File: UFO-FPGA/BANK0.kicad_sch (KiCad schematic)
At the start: 7 parts, among them U1 ICE40HX8K-BG121

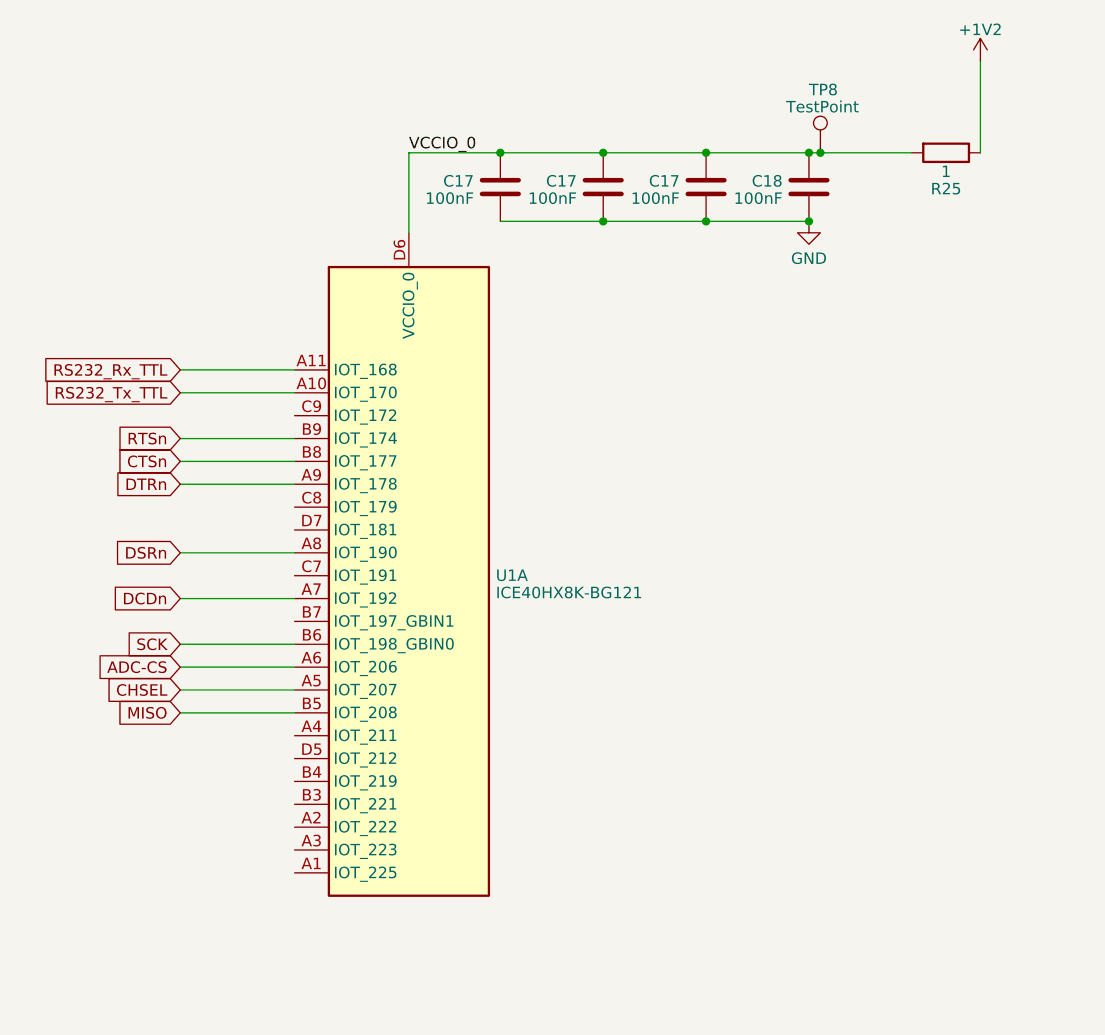
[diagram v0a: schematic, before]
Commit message: IO and power
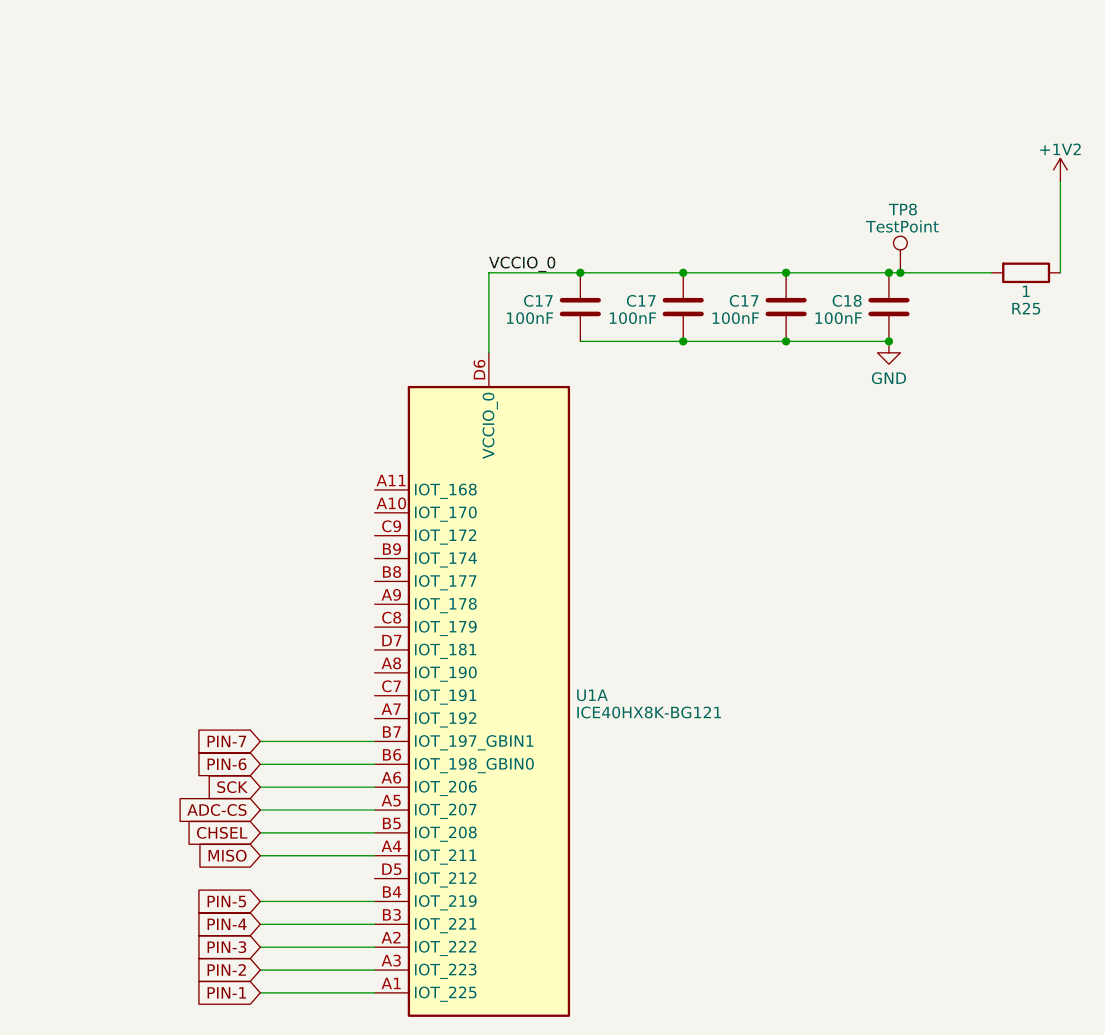
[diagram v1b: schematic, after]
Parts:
- removed C17 (x3): 100nF, symbol Device:C
- added C17 (x3): 100nF, symbol Device:C
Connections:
- net ADC-CS: now also U1.A5 (IOT_207); no longer U1.A6 (IOT_206)
- net CHSEL: now also U1.B5 (IOT_208); no longer U1.A5 (IOT_207)
- net GND: now also C17.2, C17.2, C17.2
- net MISO: now also U1.A4 (IOT_211); no longer U1.B5 (IOT_208)
- net SCK: now also U1.A6 (IOT_206); no longer U1.B6 (IOT_198_GBIN0)
- net VCCIO_0: now also C17.1, C17.1, C17.1
- net PIN-1: now reaches U1.A1 (IOT_225)
- net PIN-3: now reaches U1.A2 (IOT_222)
- net PIN-2: now reaches U1.A3 (IOT_223)
- net PIN-4: now reaches U1.B3 (IOT_221)
- net PIN-5: now reaches U1.B4 (IOT_219)
- net PIN-7: now reaches U1.B7 (IOT_197_GBIN1)
- net CTSn: no longer names the net of U1.B8 (IOT_177)
- net DCDn: no longer names the net of U1.A7 (IOT_192)
- net DSRn: no longer names the net of U1.A8 (IOT_190)
- net DTRn: no longer names the net of U1.A9 (IOT_178)
- net RS232_Rx_TTL: no longer names the net of U1.A11 (IOT_168)
- net RS232_Tx_TTL: no longer names the net of U1.A10 (IOT_170)
- net RTSn: no longer names the net of U1.B9 (IOT_174)
- new net PIN-6: U1.B6 (IOT_198_GBIN0)

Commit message: Revision
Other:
- company: (none) -> Universal-Field-Objects
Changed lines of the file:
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@@
   (paper "A4")
   (title_block
-    (date "2023-04-22")
-    (rev "V0.1")
+    (date "2023-04-25")
+    (rev "V0.5")
+    (company "Universal-Field-Objects")
   )
   (junction (at 160.02 48.895) (diameter 0) (color 0 0 0 0)

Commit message: footprints and PCB
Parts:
- R25: footprint (none) -> Resistor_SMD:R_0805_2012Metric_Pad1.20x1.40mm_HandSolder
- TP8: footprint (none) -> TestPoint:TestPoint_Keystone_5000-5004_Miniature
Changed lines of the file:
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@@
       (effects (font (size 1.27 1.27)) (justify left))
     )
-    (property "Footprint" "" (at 177.8 48.895 0)
+    (property "Footprint" "TestPoint:TestPoint_Keystone_5000-5004_Miniature" (at 177.8 48.895 0)
       (effects (font (size 1.27 1.27)) hide)
     )
@@
       (effects (font (size 1.27 1.27)))
     )
-    (property "Footprint" "" (at 186.69 47.117 90)
+    (property "Footprint" "Resistor_SMD:R_0805_2012Metric_Pad1.20x1.40mm_HandSolder" (at 186.69 47.117 90)
       (effects (font (size 1.27 1.27)) hide)
     )

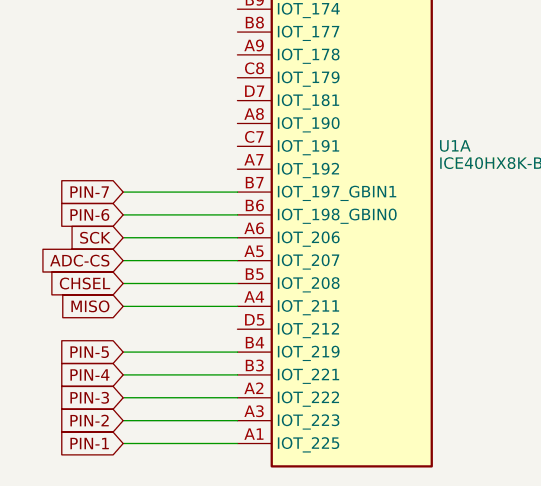
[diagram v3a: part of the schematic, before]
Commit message: footprint
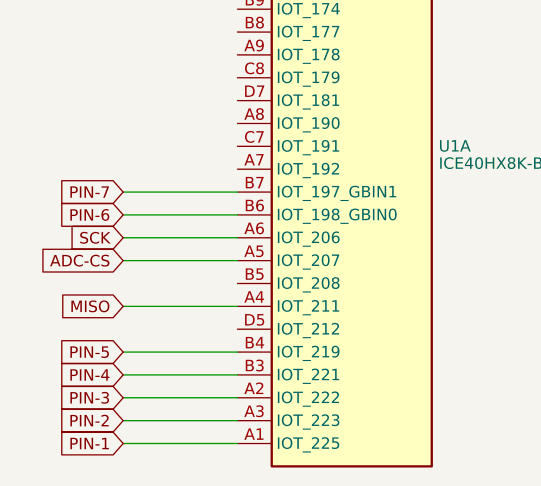
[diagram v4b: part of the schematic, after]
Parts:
- C17, C18: footprint (none) -> Capacitor_SMD:C_0805_2012Metric_Pad1.18x1.45mm_HandSolder
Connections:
- net CHSEL: no longer names the net of U1.B5 (IOT_208)
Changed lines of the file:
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@@
-    (stroke (width 0) (type default))
-  )
-  (wire (pts (xy 101.6 111.125) (xy 114.3 111.125))
     (stroke (width 0) (type default))
   )
@@
     )
   )
-  (global_label "CHSEL" (shape input) (at 101.6 111.125 180) (fields_autoplaced)
-    (effects (font (size 1.27 1.27)) (justify right))
-    (property "Intersheetrefs" "${INTERSHEET_REFS}" (at 92.7071 111.125 0)
-      (effects (font (size 1.27 1.27)) (justify right) hide)
-    )
-  )
   (global_label "PIN-2" (shape input) (at 101.6 126.365 180) (fields_autoplaced)
     (effects (font (size 1.27 1.27)) (justify right))
@@
       (effects (font (size 1.27 1.27)) (justify left))
     )
-    (property "Footprint" "" (at 147.6248 56.515 0)
+    (property "Footprint" "Capacitor_SMD:C_0805_2012Metric_Pad1.18x1.45mm_HandSolder" (at 147.6248 56.515 0)
       (effects (font (size 1.27 1.27)) hide)
     )
@@
       (effects (font (size 1.27 1.27)) (justify left))
     )
-    (property "Footprint" "" (at 159.0548 56.515 0)
+    (property "Footprint" "Capacitor_SMD:C_0805_2012Metric_Pad1.18x1.45mm_HandSolder" (at 159.0548 56.515 0)
       (effects (font (size 1.27 1.27)) hide)
     )
@@
       (effects (font (size 1.27 1.27)) (justify left))
     )
-    (property "Footprint" "" (at 170.4848 56.515 0)
+    (property "Footprint" "Capacitor_SMD:C_0805_2012Metric_Pad1.18x1.45mm_HandSolder" (at 170.4848 56.515 0)
       (effects (font (size 1.27 1.27)) hide)
     )
@@
       (effects (font (size 1.27 1.27)) (justify left))
     )
-    (property "Footprint" "" (at 136.1948 56.515 0)
-      (effects (font (size 1.27 1.27)) hide)
-    )
+    (property "Footprint" "Capacitor_SMD:C_0805_2012Metric_Pad1.18x1.45mm_HandSolder" (at 136.1948 56.515 0)
+      (effects (font (size 1.27 1.27)) hide)
+    )
